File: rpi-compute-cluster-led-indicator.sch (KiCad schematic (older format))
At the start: 29 parts, among them J1 TE_1-1734248-5_FLEX, U1 PCA9685BS,118

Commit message: Update naming convention
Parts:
- C1: footprint kvm-compute-cluster-led-indicator-footprints:0402-cap -> rpi-compute-cluster-led-indicator-footprints:0402-cap; symbol kvm-compute-cluster-led-indicator:C_100n_0402 -> rpi-compute-cluster-led-indicator:C_100n_0402
- D1, D2, D3, D4, D5: footprint kvm-compute-cluster-led-indicator-footprints:LED_Dual0603 -> rpi-compute-cluster-led-indicator-footprints:LED_Dual0603; symbol kvm-compute-cluster-led-indicator:LTST-C19HE1WT -> rpi-compute-cluster-led-indicator:LTST-C19HE1WT
- J1: footprint kvm-compute-cluster-led-indicator-footprints:TE_1-1734248-5_FLEX -> rpi-compute-cluster-led-indicator-footprints:TE_1-1734248-5_FLEX; symbol kvm-compute-cluster-led-indicator:TE_1-1734248-5_FLEX -> rpi-compute-cluster-led-indicator:TE_1-1734248-5_FLEX
- N1: footprint kvm-compute-cluster-led-indicator-footprints:antmicro-logo_scaled_15mm_silk -> rpi-compute-cluster-led-indicator-footprints:antmicro-logo_scaled_15mm_silk; symbol kvm-compute-cluster-led-indicator:antmicro_logo -> rpi-compute-cluster-led-indicator:antmicro_logo
- N2: footprint kvm-compute-cluster-led-indicator-footprints:OSHW-Logo_5.7x6mm_SilkScreen -> rpi-compute-cluster-led-indicator-footprints:OSHW-Logo_5.7x6mm_SilkScreen; symbol kvm-compute-cluster-led-indicator:oshw_logo -> rpi-compute-cluster-led-indicator:oshw_logo
- R1: footprint kvm-compute-cluster-led-indicator-footprints:0402-res -> rpi-compute-cluster-led-indicator-footprints:0402-res; symbol kvm-compute-cluster-led-indicator:R_10k_0402 -> rpi-compute-cluster-led-indicator:R_10k_0402
- R10, R13, R16, R2, R5: footprint kvm-compute-cluster-led-indicator-footprints:0402-res -> rpi-compute-cluster-led-indicator-footprints:0402-res; symbol kvm-compute-cluster-led-indicator:R_100R_0402 -> rpi-compute-cluster-led-indicator:R_100R_0402
- R11, R12, R14, R15, R17, R18, R3, R4, R6, R9: footprint kvm-compute-cluster-led-indicator-footprints:0402-res -> rpi-compute-cluster-led-indicator-footprints:0402-res; symbol kvm-compute-cluster-led-indicator:R_49R9_0402 -> rpi-compute-cluster-led-indicator:R_49R9_0402
- R19: footprint kvm-compute-cluster-led-indicator-footprints:0402-res -> rpi-compute-cluster-led-indicator-footprints:0402-res; symbol kvm-compute-cluster-led-indicator:R_0R_0402 -> rpi-compute-cluster-led-indicator:R_0R_0402
- R7, R8: footprint kvm-compute-cluster-led-indicator-footprints:0402-res -> rpi-compute-cluster-led-indicator-footprints:0402-res; symbol kvm-compute-cluster-led-indicator:R_4k7_0402 -> rpi-compute-cluster-led-indicator:R_4k7_0402
- U1: footprint kvm-compute-cluster-led-indicator-footprints:QFN-28_6x6mm_P0.65mm -> rpi-compute-cluster-led-indicator-footprints:QFN-28_6x6mm_P0.65mm; symbol kvm-compute-cluster-led-indicator:PCA9685BS,118 -> rpi-compute-cluster-led-indicator:PCA9685BS,118

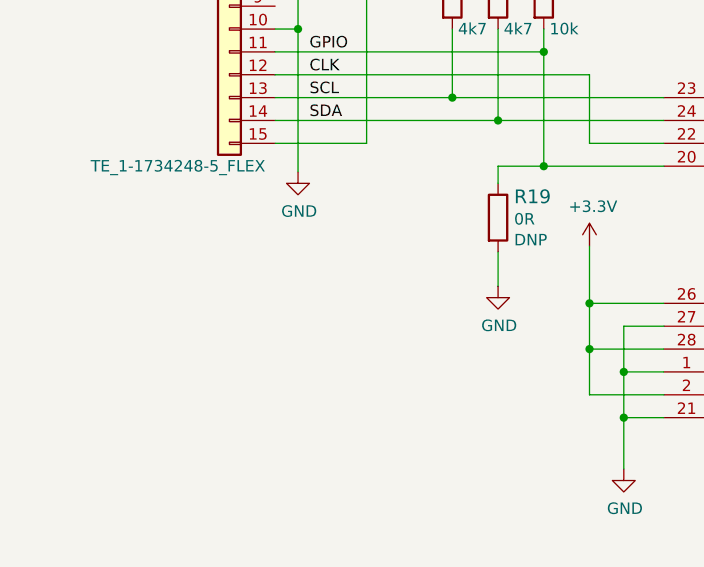
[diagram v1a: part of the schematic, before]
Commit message: Assign revision 1.1.0
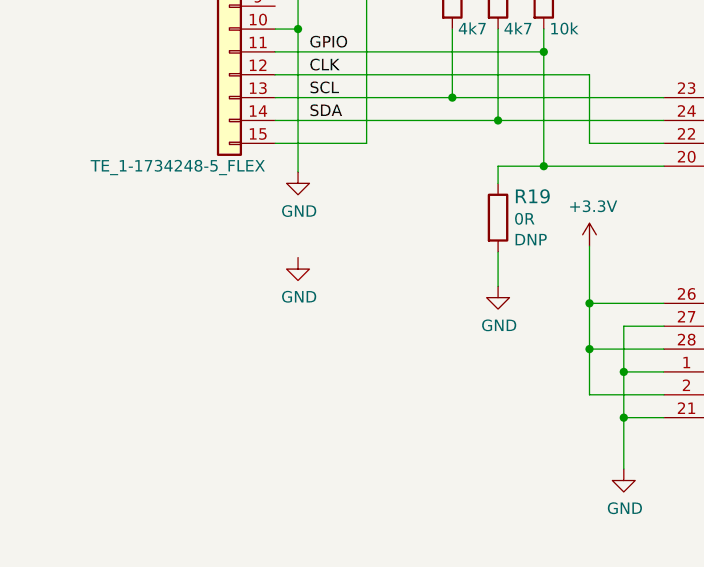
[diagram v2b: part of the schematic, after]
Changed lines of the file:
@@
 EELAYER 30 0
 EELAYER END
-$Descr A4 11693 8268
+$Descr A3 16535 11693
 encoding utf-8
 Sheet 1 1
-Title ""
-Date ""
-Rev ""
+Title "RPi Compute Cluster LED Indicator"
+Date "2022-02-18"
+Rev "1.1.0"
 Comp ""
-Comment1 ""
-Comment2 ""
+Comment1 "www.antmicro.com"
+Comment2 "Antmicro Ltd."
 Comment3 ""
 Comment4 ""
@@
 	5450 4475 5650 4475
 $Comp
-L rpi-compute-cluster-led-indicator:+3.3V #PWR0105
+L power:+3.3V #PWR0105
 U 1 1 602D0676
 P 2750 1675
@@
 	1    0    0    -1
 $EndComp
+$Comp
+L power:GND #PWR?
+U 1 1 62103425
+P 2450 3675
+F 0 "#PWR?" H 2450 3425 50  0001 C CNN
+F 1 "GND" H 2455 3502 50  0000 C CNN
+F 2 "" H 2450 3675 50  0001 C CNN
+F 3 "" H 2450 3675 50  0001 C CNN
+	1    2450 3675
+	1    0    0    -1
+$EndComp
